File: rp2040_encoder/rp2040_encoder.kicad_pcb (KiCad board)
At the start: 2 copper layers, 36.7 x 33.3 mm, 15 parts, among them J1 Conn_01x02, J2 Conn_01x06, U5 MT6701

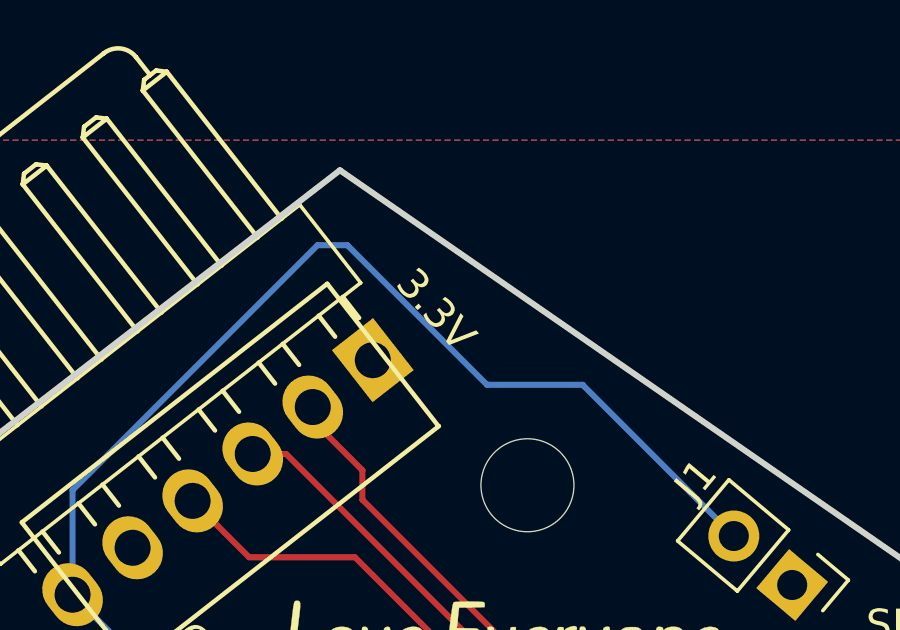
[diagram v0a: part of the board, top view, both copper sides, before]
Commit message: Updated files for boards ordered July 2024
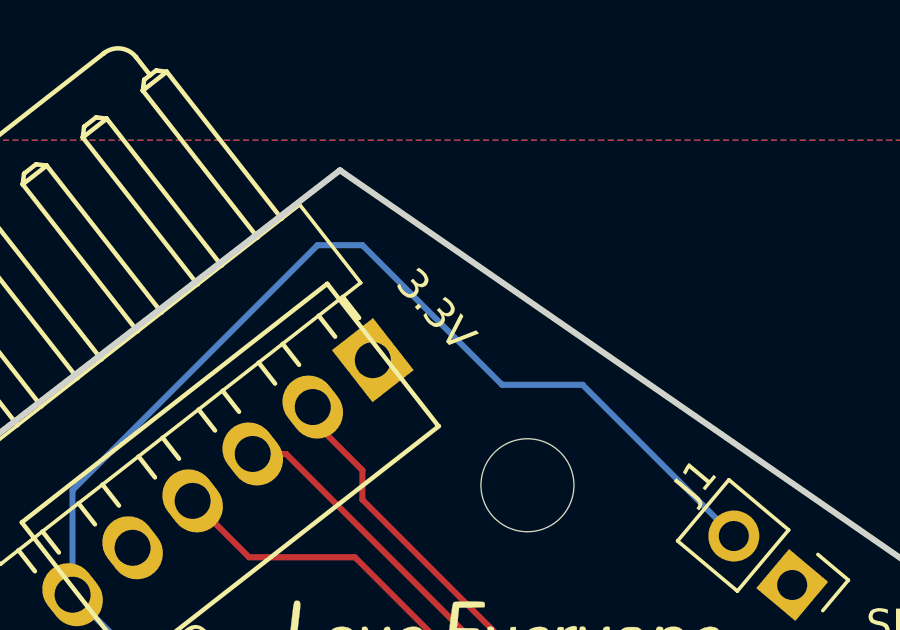
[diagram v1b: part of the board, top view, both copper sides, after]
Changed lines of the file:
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@@
 	)
 	(paper "A4")
+	(title_block
+		(title "rp2040_encoder")
+	)
 	(layers
 		(0 "F.Cu" signal)
@@
 			(net 6 "unconnected-(U5-OUT-Pad3)")
 			(pinfunction "OUT")
-			(pintype "output")
+			(pintype "output+no_connect")
 		)
 		(pad "4" smd roundrect
@@
 			(net 7 "unconnected-(U5-PUSH-Pad5)")
 			(pinfunction "PUSH")
-			(pintype "output")
+			(pintype "output+no_connect")
 		)
 		(pad "6" smd roundrect
@@
 	)
 	(gr_circle
-		(center 142.5 95)
-		(end 142.5 94.5)
+		(center 150 100)
+		(end 150 99.5)
 		(stroke
 			(width 0.1)
@@
 	)
 	(segment
-		(start 144 82.5)
-		(end 143 82.5)
+		(start 136.188362 95.5)
+		(end 134.837263 94.148901)
 		(width 0.2)
 		(layer "B.Cu")
@@
 	)
 	(segment
-		(start 136.188362 95.5)
-		(end 134.837263 94.148901)
+		(start 156.879248 92.192319)
+		(end 151.836929 87.15)
 		(width 0.2)
 		(layer "B.Cu")
@@
 	)
 	(segment
-		(start 148.65 87.15)
-		(end 144 82.5)
+		(start 149.15 87.15)
+		(end 144.5 82.5)
 		(width 0.2)
 		(layer "B.Cu")
@@
 	)
 	(segment
-		(start 148.5 104.5)
-		(end 146.61005 104.5)
+		(start 134.837263 90.662737)
+		(end 134.837263 94.148901)
 		(width 0.2)
 		(layer "B.Cu")
@@
 	)
 	(segment
-		(start 143 82.5)
-		(end 134.837263 90.662737)
+		(start 151.836929 87.15)
+		(end 149.15 87.15)
 		(width 0.2)
 		(layer "B.Cu")
@@
 	)
 	(segment
-		(start 156.879248 92.192319)
-		(end 151.836929 87.15)
+		(start 144.5 82.5)
+		(end 143 82.5)
 		(width 0.2)
 		(layer "B.Cu")
@@
 	)
 	(segment
-		(start 134.837263 90.662737)
-		(end 134.837263 94.148901)
+		(start 143 82.5)
+		(end 134.837263 90.662737)
+		(width 0.2)
+		(layer "B.Cu")
+		(net 11)
+	)
+	(segment
+		(start 148.5 104.5)
+		(end 146.61005 104.5)
 		(width 0.2)
 		(layer "B.Cu")
@@
 		(width 0.2)
 		(layer "B.Cu")
-		(net 11)
-	)
-	(segment
-		(start 151.836929 87.15)
-		(end 148.65 87.15)
-		(width 0.2)
-		(layer "B.Cu")
